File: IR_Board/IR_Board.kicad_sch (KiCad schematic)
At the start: 64 parts, among them J1 CONN_OUT, Q1 FDG6335N, Q10 FDG6335N, Q11 FDG6335N, Q12 FDG6335N, Q13 FDG6335N, Q14 FDG6335N, Q2 FDG6335N, Q3 FDG6335N, Q4 FDG6335N, Q5 FDG6335N, Q6 FDG6335N, Q7 FDG6335N, Q8 FDG6335N, Q9 FDG6335N, SW1 SW_SPDT, U1 TSSP58038, U10 TSSP58038, U11 TSSP58038, U12 TSSP58038, U13 TSSP58038, U14 TSSP58038, U2 TSSP58038, U3 TSSP58038, U4 TSSP58038, U5 TSSP58038, U6 TSSP58038, U7 TSSP58038, U8 TSSP58038, U9 TSSP58038

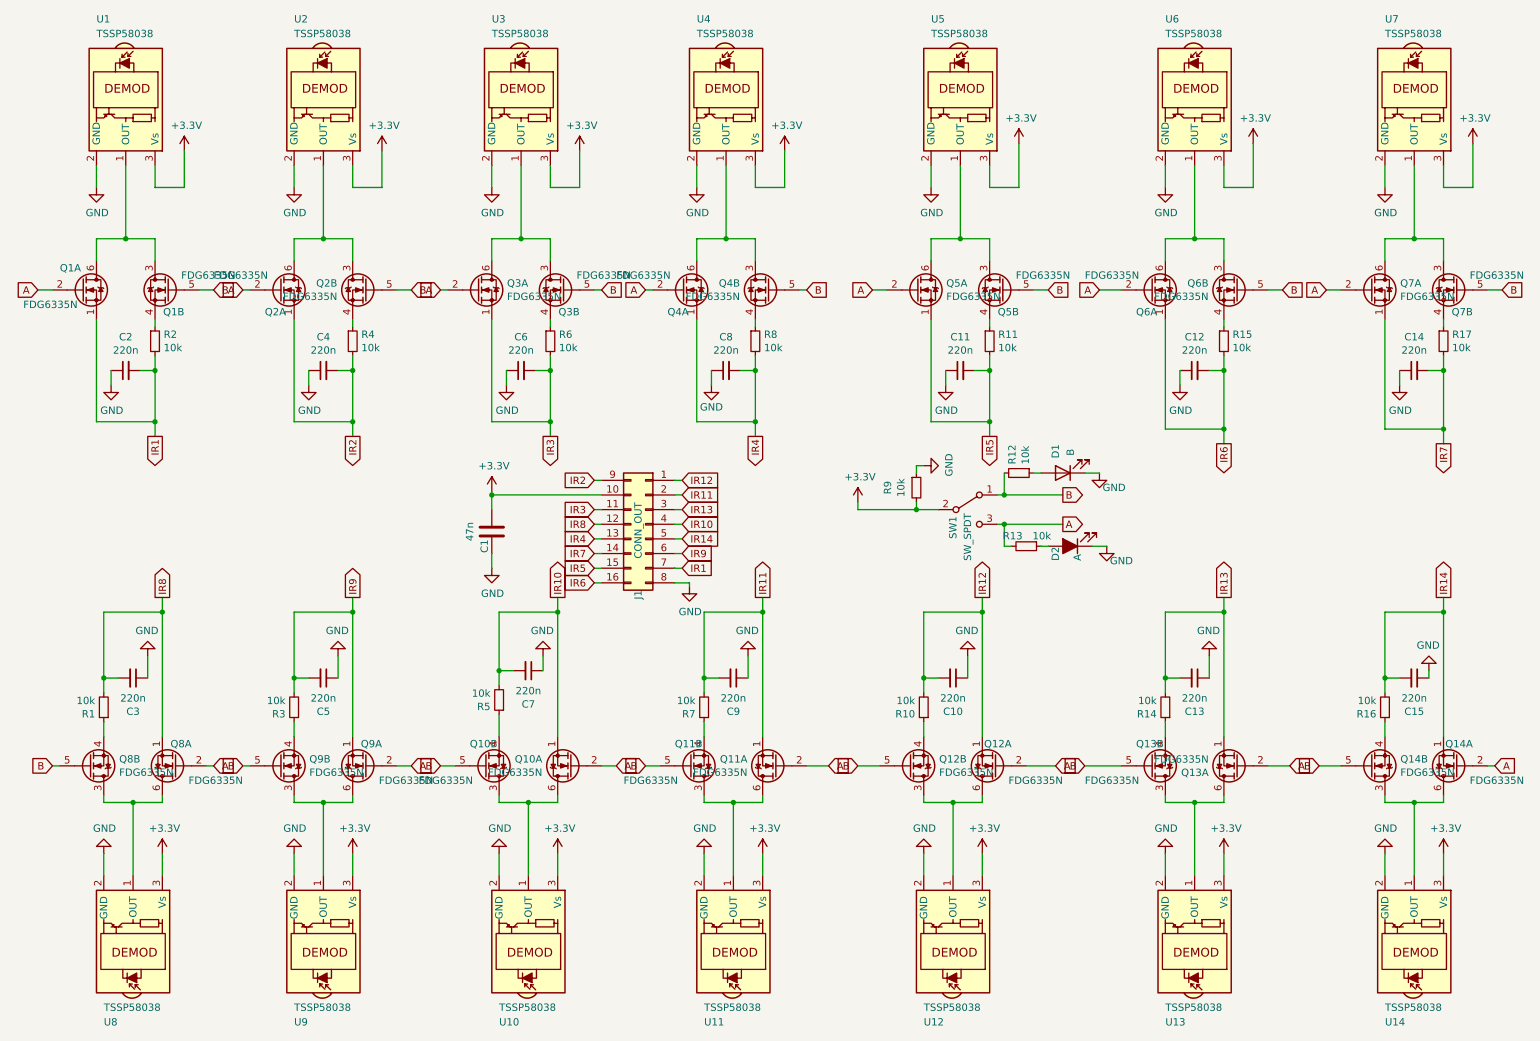
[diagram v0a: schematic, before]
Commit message: Finished IR, generated gerbers, ordered designs
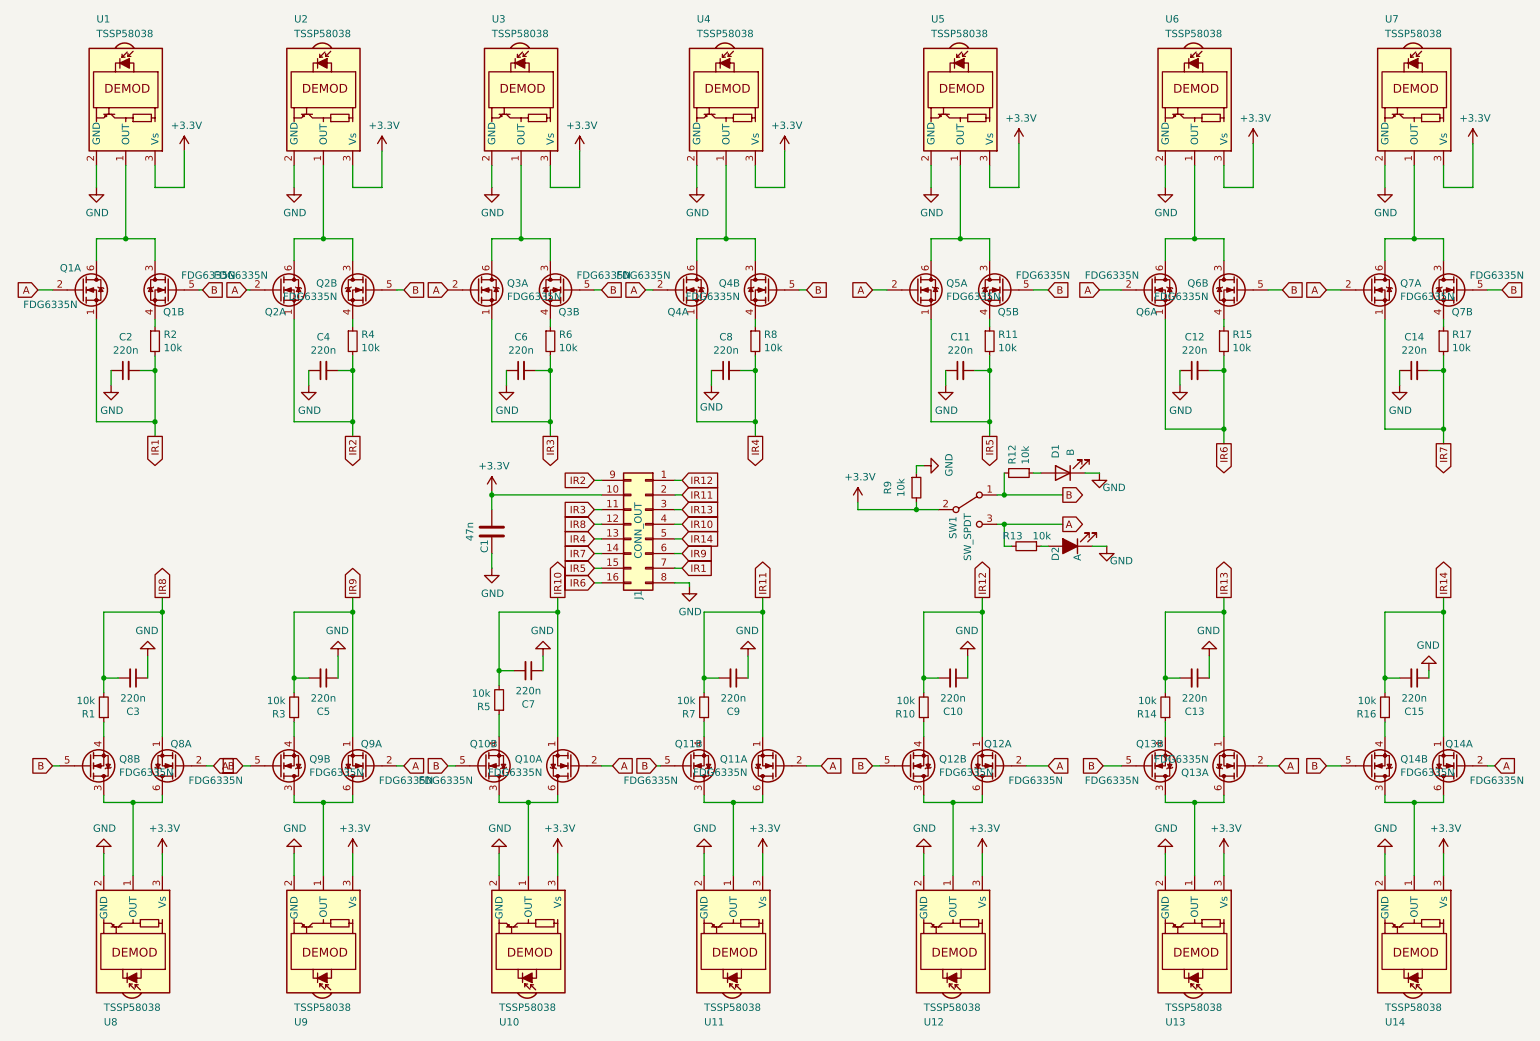
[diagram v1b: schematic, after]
